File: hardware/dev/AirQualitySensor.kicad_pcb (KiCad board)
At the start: 2 copper layers, 81.3 x 36.8 mm, 44 parts, among them J1 USB_C_Receptacle_USB2.0, J2 SWD, J3 UART, U1 004-0-0053, U2 DHT22, U3 XC6206P332MR

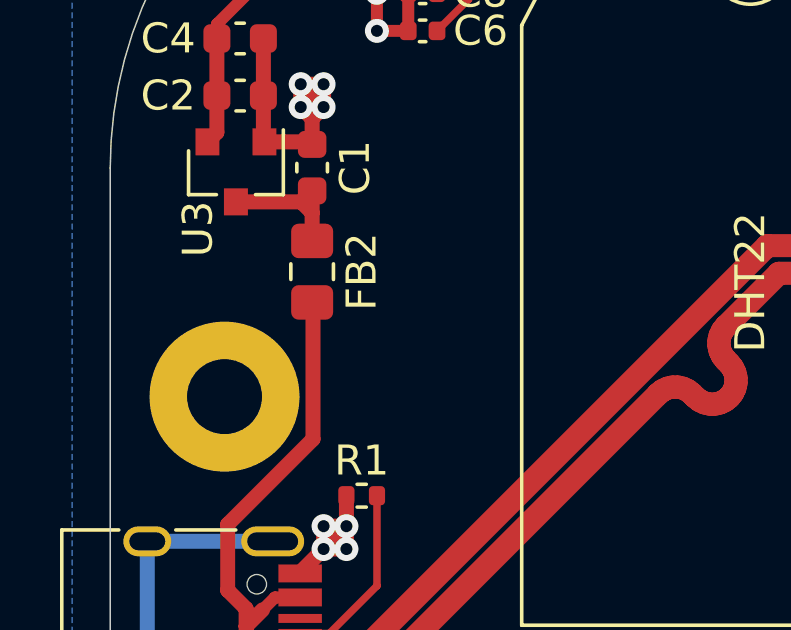
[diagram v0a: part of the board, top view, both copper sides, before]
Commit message: Fix clearance issue
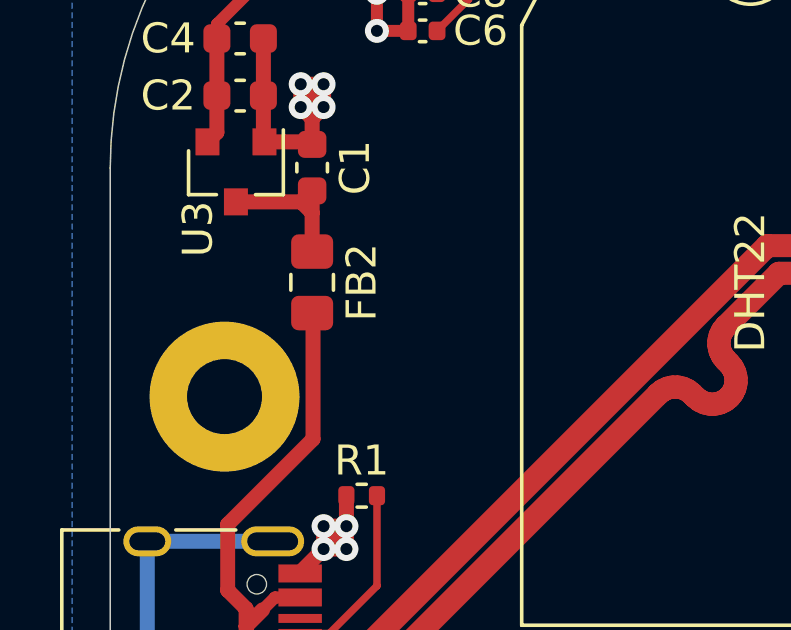
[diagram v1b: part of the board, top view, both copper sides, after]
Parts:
- moved FB2 0.36 mm to (113.4, 102.9)
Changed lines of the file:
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@@
     (thickness 1.6)
     (drawings 24)
-    (tracks 586)
+    (tracks 587)
     (zones 0)
     (modules 44)
@@
   )
   (setup
-    (last_trace_width 0.25)
+    (last_trace_width 0.5)
     (user_trace_width 0.4)
     (user_trace_width 0.5)
@@
   )
   (module Inductor_SMD:L_0805_2012Metric_Pad1.15x1.40mm_HandSolder (layer F.Cu)
-    (at 113.411 102.5145 270)
+    (at 113.411 102.87 270)
     (descr "Inductor SMD 0805 (2012 Metric), square (rectangular) end terminal, IPC_7351 nominal with elongated pad for handsoldering. (Body size source: https://docs.google.com/spreadsheets/d/1BsfQQcO9C6DZCsRaXUlFlo91Tg2WpOkGARC1WS5S8t0/edit?usp=sharing), generated with kicad-footprint-generator")
     (tags "inductor handsolder")
@@
   (segment (start 111.20999 114.33501) (end 111.20999 113.74999) (width 0.5) (layer F.Cu) (net 26))
   (segment (start 113.440001 103.606001) (end 113.411 103.577) (width 0.5) (layer F.Cu) (net 26))
-  (segment (start 113.440001 108.096001) (end 113.440001 103.606001) (width 0.5) (layer F.Cu) (net 26))
   (segment (start 121.92 121.142006) (end 121.912003 121.150003) (width 0.5) (layer F.Cu) (net 26))
   (segment (start 121.92 120.9505) (end 121.92 121.142006) (width 0.5) (layer F.Cu) (net 26))
+  (segment (start 113.440001 103.924001) (end 113.411 103.895) (width 0.5) (layer F.Cu) (net 26))
+  (segment (start 113.440001 108.096001) (end 113.440001 103.924001) (width 0.5) (layer F.Cu) (net 26))
   (segment (start 113.046 100.187) (end 113.411 99.822) (width 0.5) (layer F.Cu) (net 27))
   (segment (start 110.871 100.187) (end 113.046 100.187) (width 0.5) (layer F.Cu) (net 27))
   (segment (start 113.411 100.552) (end 113.046 100.187) (width 0.5) (layer F.Cu) (net 27))
-  (segment (start 113.411 99.822) (end 113.411 101.452) (width 0.5) (layer F.Cu) (net 27))
+  (segment (start 113.411 99.822) (end 113.411 101.845) (width 0.5) (layer F.Cu) (net 27))
   (segment (start 115.572 112.988) (end 115.572 109.982) (width 0.25) (layer F.Cu) (net 29))
   (segment (start 113.986 114.574) (end 115.572 112.988) (width 0.25) (layer F.Cu) (net 29))
